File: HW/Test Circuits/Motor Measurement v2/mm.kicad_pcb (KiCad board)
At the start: 2 copper layers, 49 parts, among them J1 IN, J2 MOTOR, J3 PWR, J4 OUT, J5 CONN_9X2, U1 MCP6002, U2 MCP6002

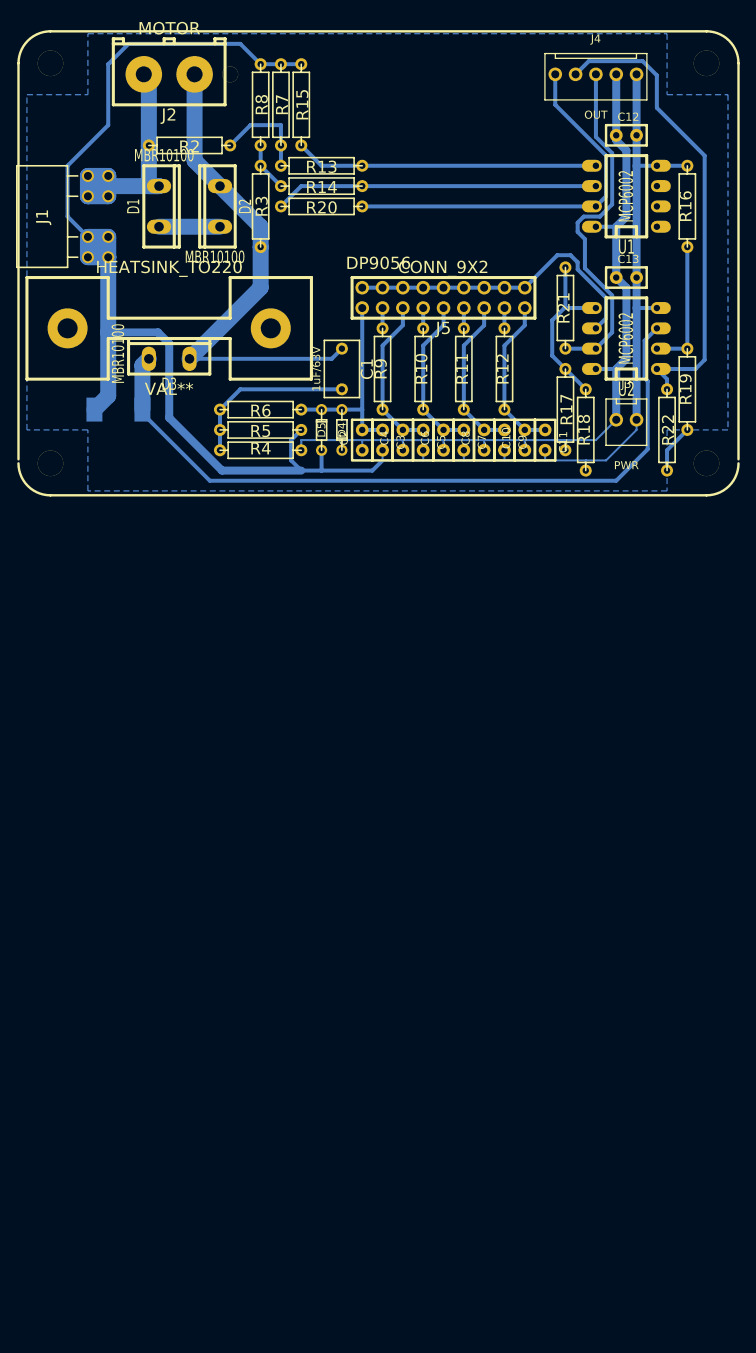
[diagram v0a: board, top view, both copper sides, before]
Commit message: Motor Measurement v2 cleanup
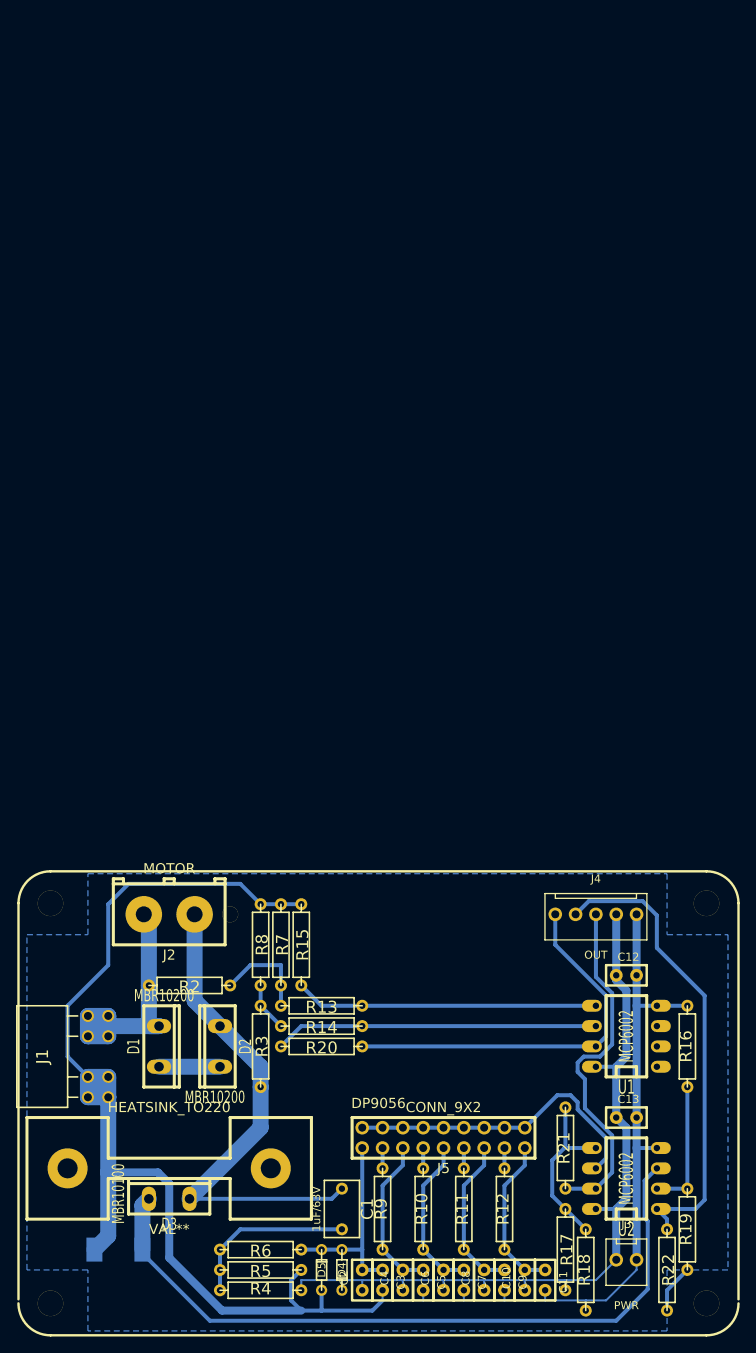
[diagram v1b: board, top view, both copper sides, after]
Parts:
- D1, D2: value MBR10100 -> MBR10200
- R8: value 21K -> 1K1
- moved J5 105.0 mm to (80.0, 159.6)
- moved R1 105.0 mm to (39.4, 173.6)
- moved R17 105.0 mm to (95.2, 173.6)
- moved R6 105.0 mm to (57.1, 173.6)
- moved C1 105.0 mm to (67.3, 168.5)
- moved C12 105.0 mm to (102.9, 139.3)
- moved C13 105.0 mm to (102.9, 157.1)
- moved D1 105.0 mm to (44.5, 148.2)
- moved D2 105.0 mm to (52.1, 148.2)
- moved D3 105.0 mm to (45.7, 167.2)
- moved D4 105.0 mm to (67.3, 176.1)
- moved D5 105.0 mm to (64.8, 176.1)
- moved DP9056 105.0 mm to (71.9, 155.3)
- moved J3 105.0 mm to (102.9, 174.8)
- moved R10 105.0 mm to (77.5, 168.5)
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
